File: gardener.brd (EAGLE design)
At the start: 73.5 x 55 mm, 40 parts, among them IC1 AMS1117, IC2 AMS1117

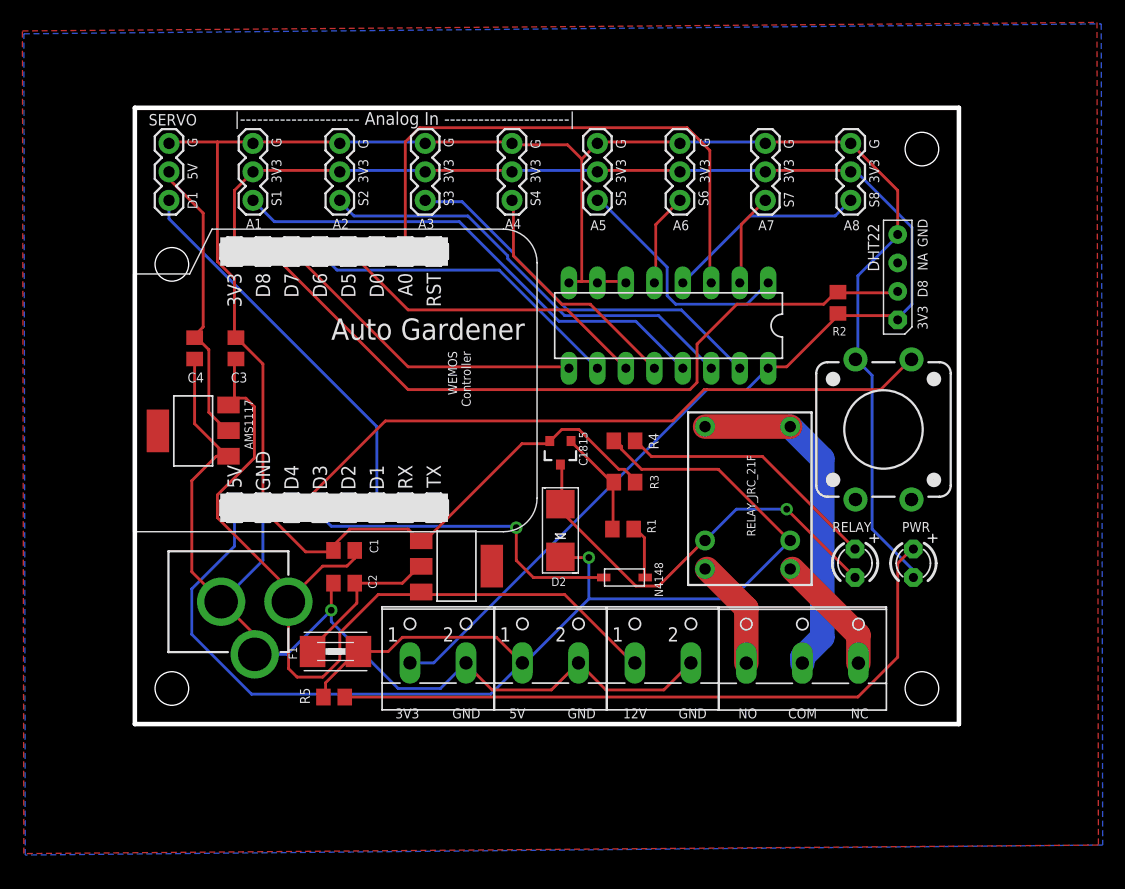
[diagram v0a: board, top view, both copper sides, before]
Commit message: Update design to version 0.2
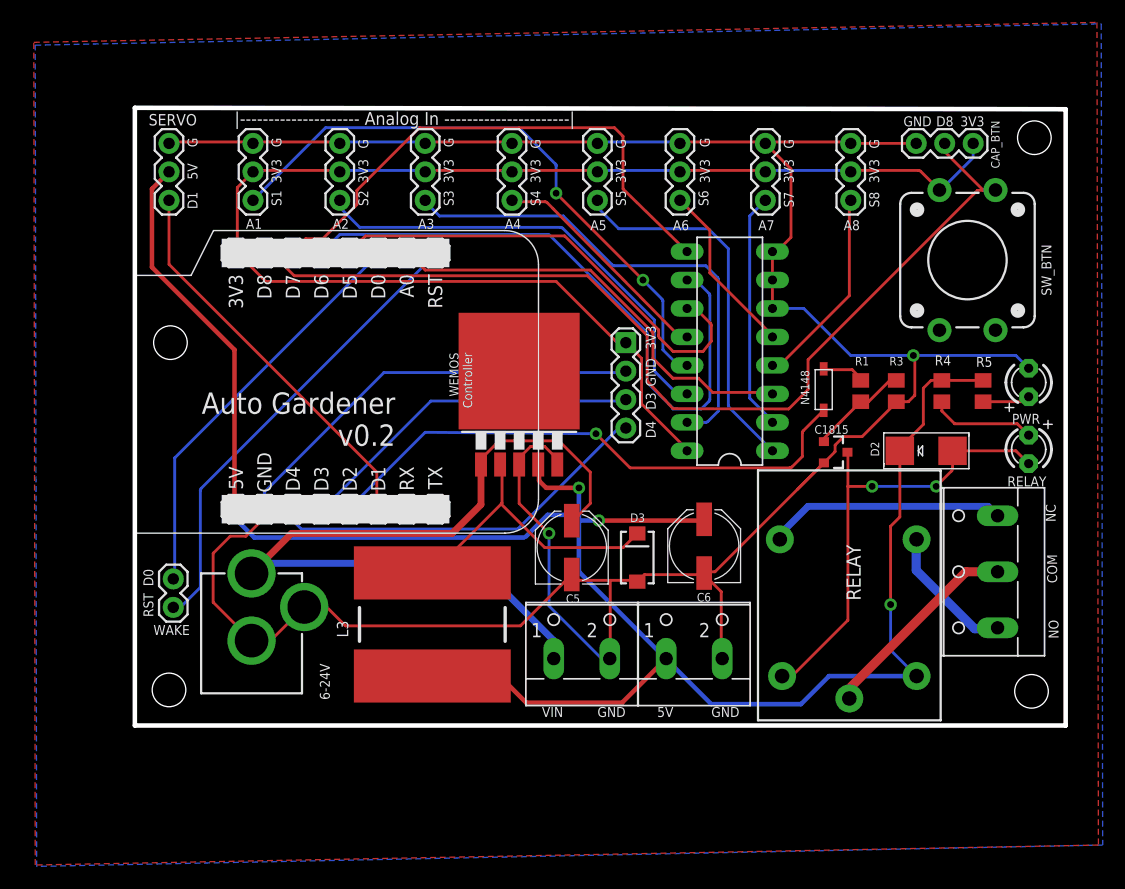
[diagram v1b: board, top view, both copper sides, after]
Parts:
- removed C1, C3: 100uF, rcl:C0805
- removed C2, C4: 22uF, rcl:C0805
- removed DHT22: (no value), RHT03_DHT-22_AM2302:AM2302
- removed F1: 1A/15V, adafruit:1812
- removed IC1, IC2: AMS1117, burr-brown:SOT223
- removed JP1: POWER IN 6-12V, SparkFun-Connectors:POWER_JACK_PTH
- removed R2: 10K, rcl:R0805
- removed S2: SWITCH-MOMENTARY-212MM, SparkFun-Electromechanical:TACTILE-PTH-12MM
- removed U$4: RELAY_JRC_21F, My Eagle Lib:MINIATURE_RELAY_JRC_21F
- removed X4: (no value), con-wago-500:W237-102
- added C5, C6: 100uF/35V, SparkFun-Passives:PANASONIC_D
- added CAP_BTN: (no value), SparkFun-Connectors:1X03
- added D3: SS34, SparkFun-DiscreteSemi:SMA-DIODE
- added IC4: LM2596S, national-semiconductor:TO263-5
- added JP2: POWER IN, SparkFun-Connectors:POWER_JACK_PTH
- added L3: 100uH, SparkFun-Passives:INDUCTOR_SDR1307
- added OLED: (no value), SparkFun-Connectors:1X04
- added RELAY: ZNS5106, relay:ZN5
- added SW_BTN: SWITCH-MOMENTARY-212MM, SparkFun-Electromechanical:TACTILE-PTH-12MM
- added WAKE: (no value), SparkFun-Connectors:1X02
- moved R5 64.0 mm to (75.9, 29.3), turned to 270 degrees
- moved D2 33.4 mm to (70.9, 24.0), turned to 0 degrees
- moved R4 28.7 mm to (72.3, 29.3), turned to 270 degrees
- moved R3 25.6 mm to (68.2, 29.3), turned to 90 degrees
- moved R1 24.5 mm to (65.0, 29.3), turned to 270 degrees
- moved C1815 24.5 mm to (62.7, 23.9), turned to 270 degrees
- moved N4148 24.4 mm to (61.7, 29.5), turned to 270 degrees
- moved LED2 19.1 mm to (80.0, 30.1), turned to 90 degrees
- moved LED1 18.5 mm to (80.0, 24.1)
- moved X1 17.5 mm to (75.9, 13.2), turned to 90 degrees
- moved X3 12.8 mm to (50.2, 6.73)
- moved U$2 10.1 mm to (80.5, 51.9)
- moved U$6 9.78 mm to (80.3, 2.54)
- moved X2 7.25 mm to (40.1, 6.73)
- moved U$5 6.99 mm to (3.43, 33.7)
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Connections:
- removed net 5V_MOTOR: C4.1, IC1.2, SERVO.2
- removed net VOUT: C2.1, F1.1, IC2.2
- new net N$9: D3.C, IC4.2, L3.P$1
- new net RST: U$3.RST, WAKE.1
- net +3V3: now also CAP_BTN.3, OLED.1, SW_BTN.3; no longer DHT22.VDD, R2.1, X4.1
- net 5V: now also C6.+, IC4.4, L3.P$2, RELAY.A1, SERVO.2; no longer F1.2, U$4.COIL1
- net COM: now also RELAY.11; no longer U$4.COM1, U$4.COM2
- net D0: now also WAKE.2
- net D2: now also N4148.A
- net D3: now also OLED.3; no longer N4148.A
- net D4: now also OLED.4; no longer S2.1
- net D8: now also CAP_BTN.2, SW_BTN.1; no longer DHT22.DATA, R2.2
- net GND: now also C5.-, C6.-, CAP_BTN.1, D3.A, IC4.3, IC4.5, JP2.GND, JP2.GNDBREAK, OLED.2; no longer C1.2, C2.2, C3.2, C4.2, DHT22.GND, IC1.1, IC2.1, JP1.GND, JP1.GNDBREAK, S2.3, X4.2
- net N$1: now also RELAY.A2; no longer U$4.COIL2
- net NC: now also RELAY.12; no longer U$4.NC
- net NO: now also RELAY.14; no longer U$4.NO
- net VIN: now also C5.+, IC4.1, JP2.PWR; no longer C1.1, C3.1, IC1.3, IC2.3, JP1.PWR
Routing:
- net 5V: track 121.8 -> 184.1 mm, vias 1 -> 3
- net N$4: track 61.1 -> 4.25 mm
- net D2: track 0.00 -> 49.9 mm, vias 0 -> 1
- net RST: track 0.00 -> 41.5 mm
- net D0: track 0.00 -> 36.5 mm
- net D6: track 29.0 -> 56.8 mm
- net N$9: track 0.00 -> 26.9 mm
- net 5V_MOTOR: track 26.2 -> 0.00 mm
- net D4: track 60.7 -> 34.9 mm
- net D8: track 67.8 -> 89.7 mm
- net D7: track 29.1 -> 47.8 mm
- net VOUT: track 14.5 -> 0.00 mm
- net N$3: track 23.6 -> 9.47 mm
- net GND: track 296.0 -> 282.9 mm, vias 1 -> 2
- net D5: track 29.1 -> 42.1 mm
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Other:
- board size 73.5 x 55 mm -> 83.1 x 55.1 mm
- board text added: "6-24V"
- board text added: "Auto Gardener v0.2"
- board text added: "D0"
- board text added: "D3"
- board text added: "D4"
- board text added: "RST"
- board text added: "SW_BTN"
- board text added: "VIN"
- board text removed: "12V"
- board text removed: "Auto Gardener"
- board text removed: "NA"
